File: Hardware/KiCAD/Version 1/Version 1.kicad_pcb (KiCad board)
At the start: 2 copper layers, 199 x 99 mm, 41 parts, among them J1 Conn_01x03_Pin, J10 Conn_01x03_Pin, J11 Conn_01x03_Pin, J12 Conn_01x03_Pin, J13 Conn_01x03_Pin, J14 Conn_01x03_Pin, J15 Conn_01x03_Pin, J16 Conn_01x03_Pin, J17 Conn_01x02_Pin, J2 Conn_01x03_Pin, J3 Conn_01x03_Pin, J4 Conn_01x03_Pin, J5 Conn_01x03_Pin, J6 Conn_01x03_Pin, J7 Conn_01x03_Pin, J8 Conn_01x03_Pin, J9 Conn_01x03_Pin, SW1 Button 1, SW2 Button 2, SW3 Button 3, SW4 Button 4, SW5 Button 5

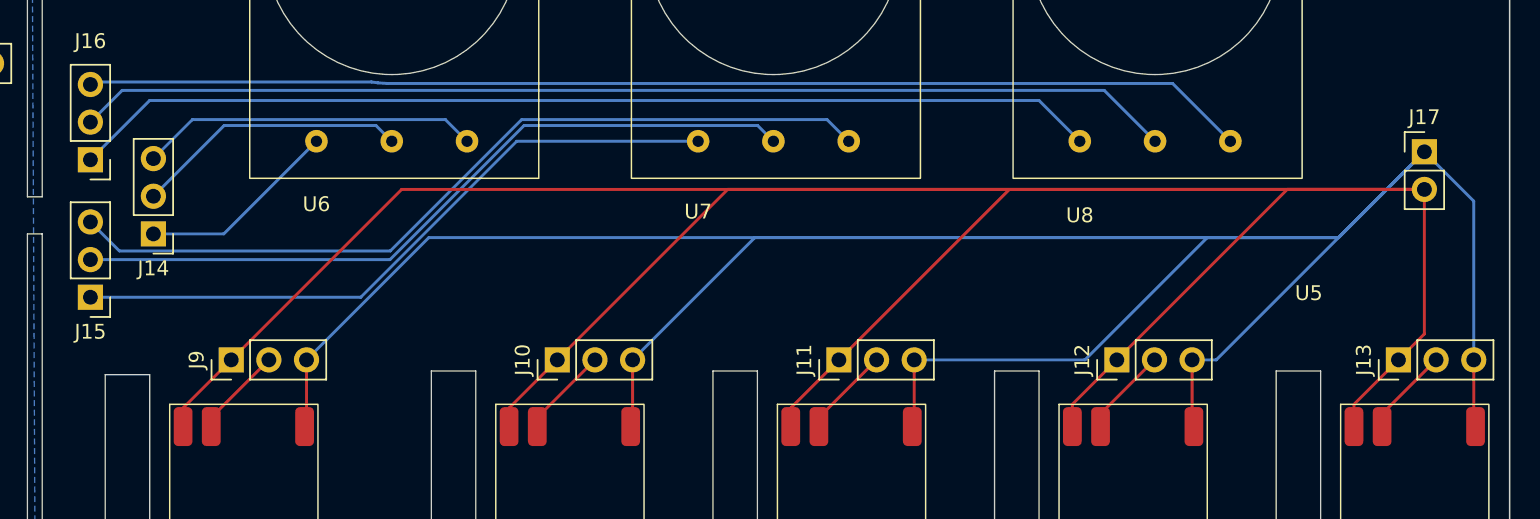
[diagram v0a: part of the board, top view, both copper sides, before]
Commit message: to be ordererd
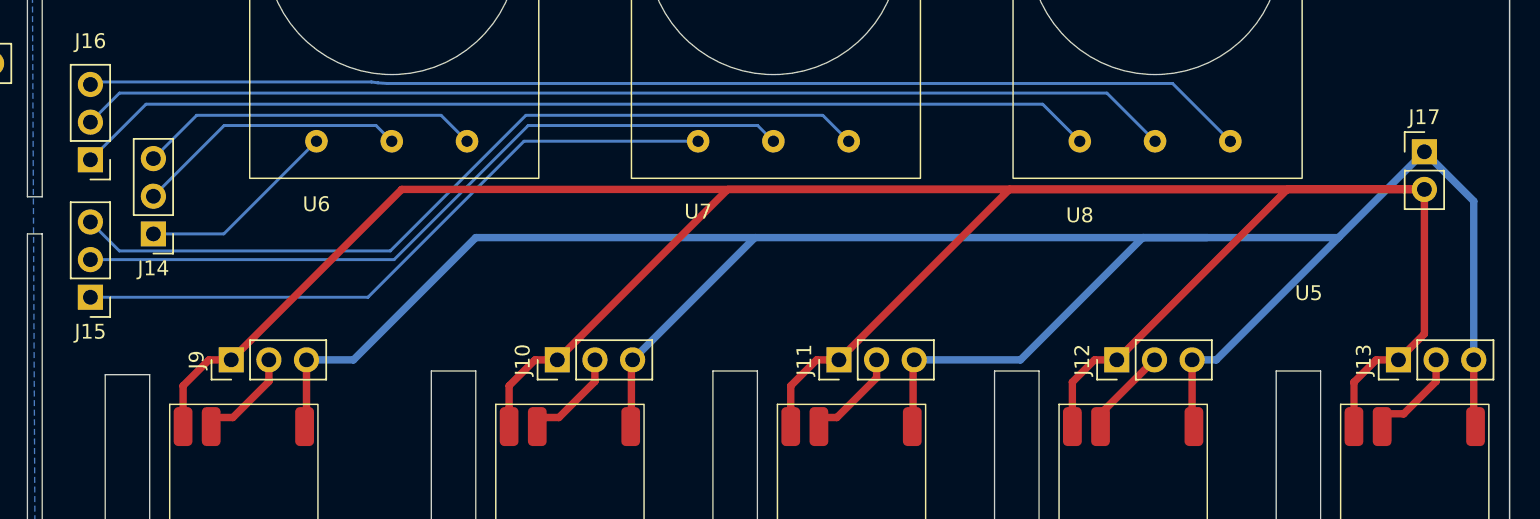
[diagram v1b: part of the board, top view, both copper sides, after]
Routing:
- net Net-(J10-Pin_1): track 259.6 -> 263.9 mm
- net Net-(J9-Pin_2): track 6.11 -> 6.97 mm
- net Net-(J10-Pin_2): track 6.11 -> 6.97 mm
- net Net-(J13-Pin_2): track 6.01 -> 6.86 mm
- net Net-(J11-Pin_2): track 6.11 -> 6.82 mm
